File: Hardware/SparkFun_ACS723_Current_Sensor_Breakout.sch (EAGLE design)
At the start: 19 parts, among them J1 455-1750-1-ND, U1 ACS723

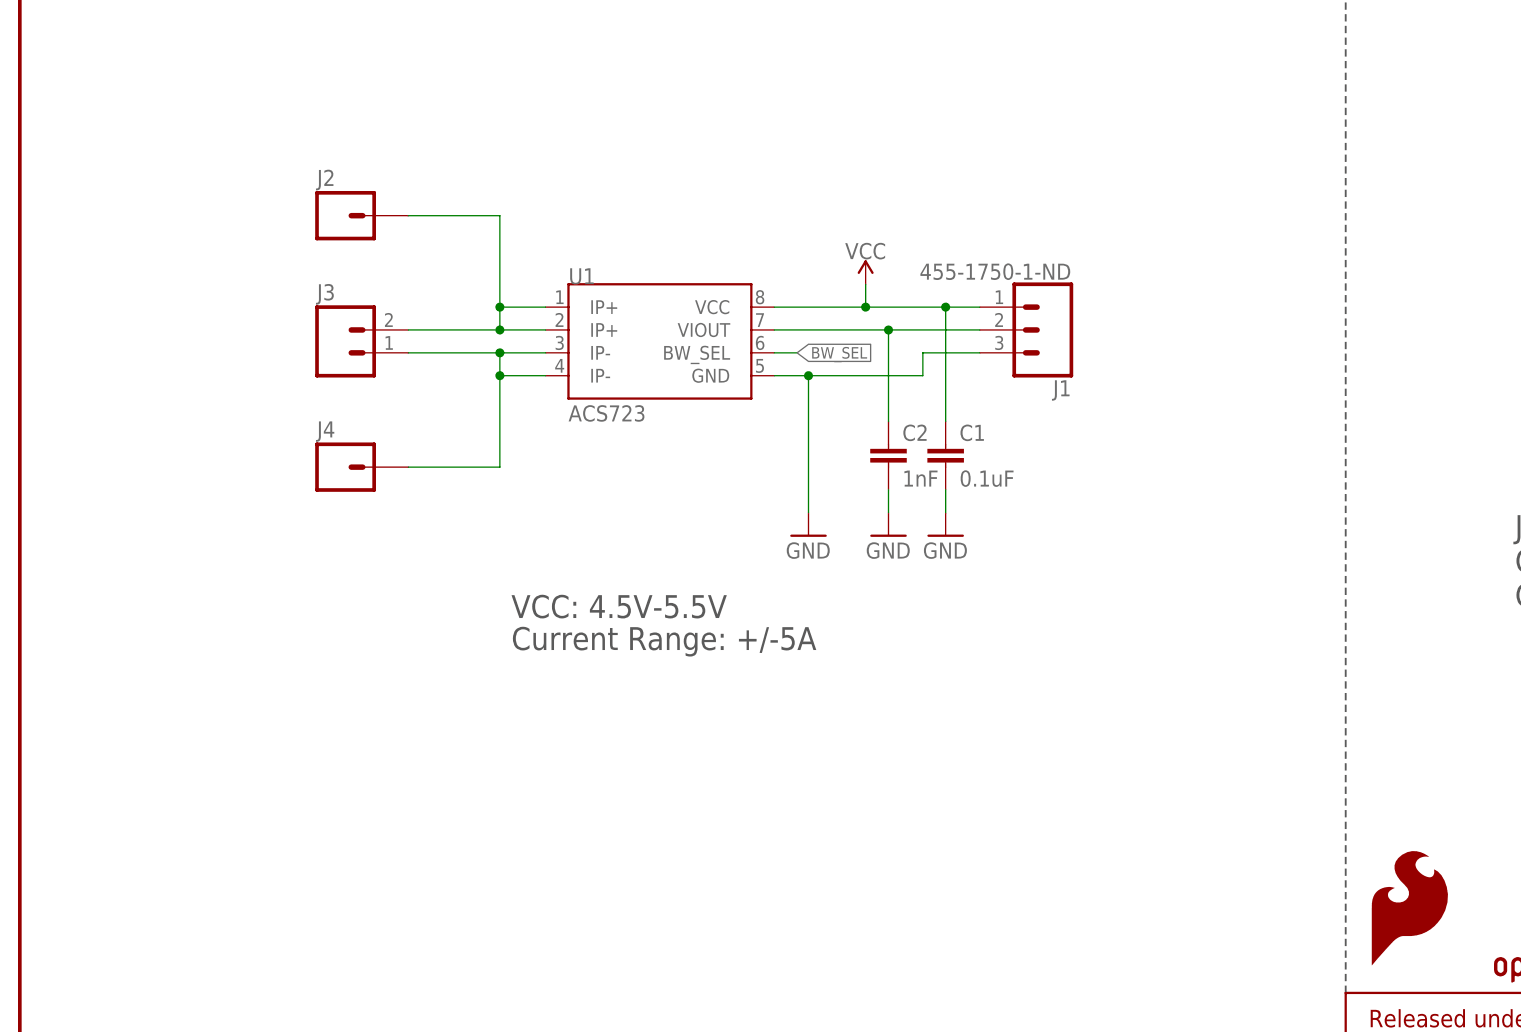
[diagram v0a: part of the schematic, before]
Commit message: removed old design files
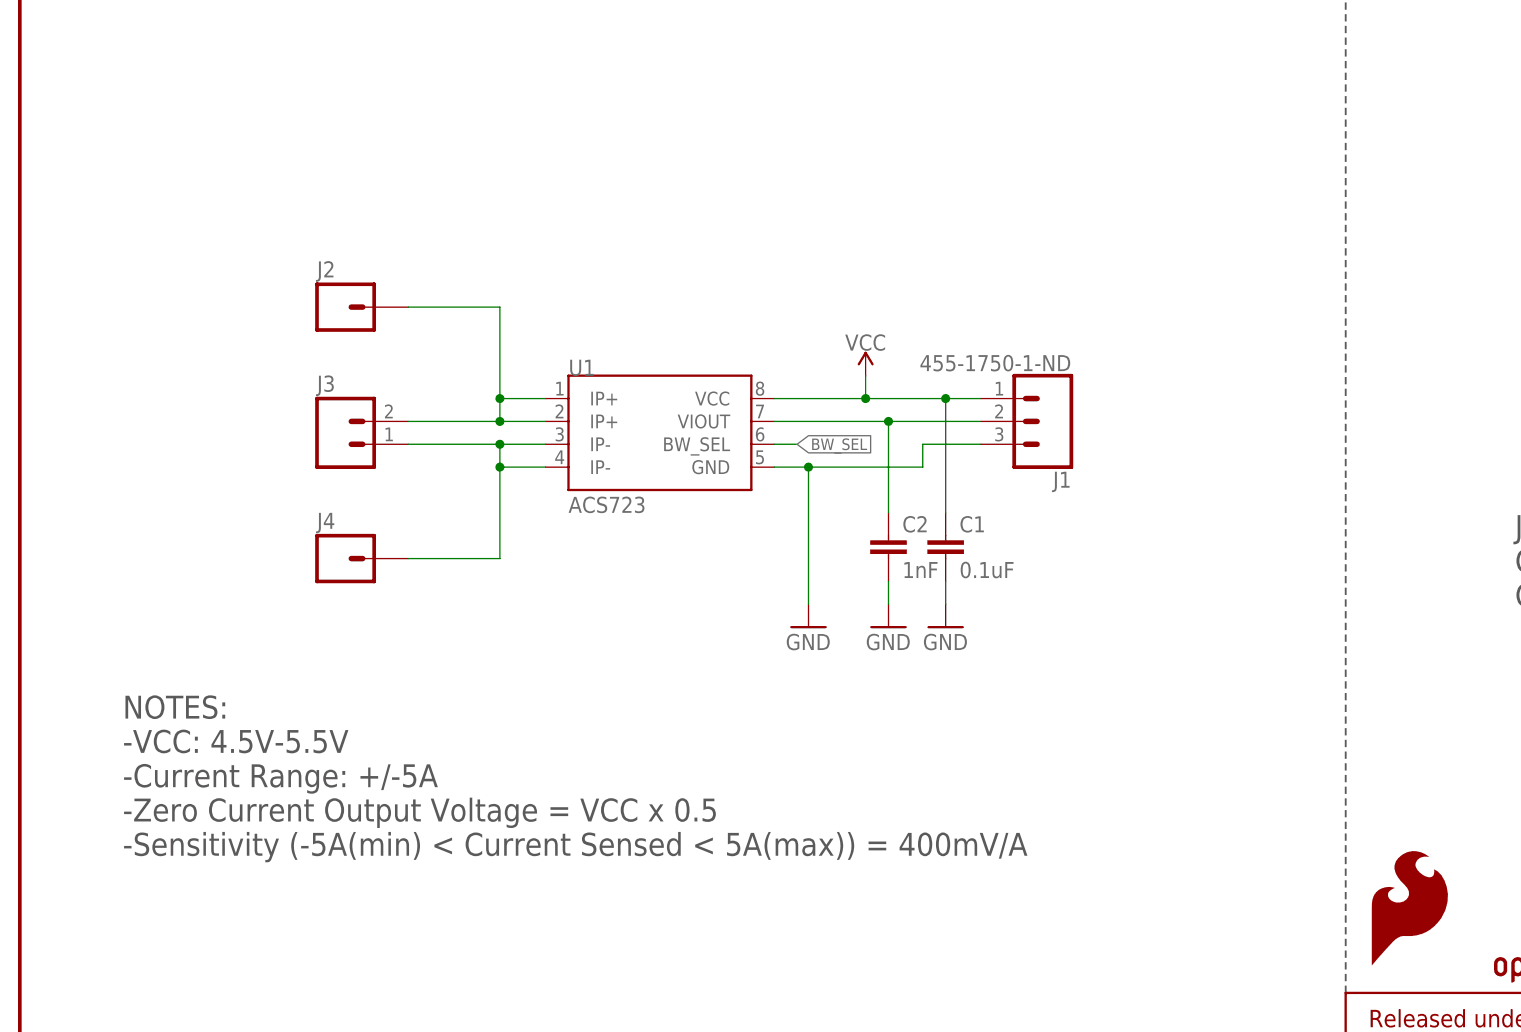
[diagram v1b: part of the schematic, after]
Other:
- note added: "-Current Range: +/-5A"
- note added: "-Sensitivity (-5A(min) < Current Sensed < 5A(max)) = 400mV/A"
- note added: "-VCC: 4.5V-5.5V"
- note added: "-Zero Current Output Voltage = VCC x 0.5"
- note added: "NOTES:"
- note removed: "Current Range: +/-5A"
- note removed: "VCC: 4.5V-5.5V"
- moved on the sheet: C1, C2, J1, J2, J3, J4, U1
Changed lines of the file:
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@@
 <text x="236.982" y="7.366" size="2.54" layer="94">v10</text>
 <text x="175.26" y="6.604" size="2.54" layer="94">Eric Orosel</text>
-<text x="54.61" y="73.66" size="2.54" layer="97">Current Range: +/-5A</text>
-<text x="54.61" y="77.216" size="2.54" layer="97">VCC: 4.5V-5.5V</text>
+<text x="11.43" y="58.42" size="2.54" layer="97">-Current Range: +/-5A</text>
+<text x="11.43" y="62.23" size="2.54" layer="97">-VCC: 4.5V-5.5V</text>
 <text x="166.116" y="86.106" size="2.54" layer="97">JP1 (Sets bandwidth):</text>
 <text x="166.116" y="78.486" size="2.54" layer="97">CLOSED = 80kHz</text>
@@
 <text x="2.286" y="180.34" size="2.54" layer="97">ACS723LLCTR-05AB-T2</text>
 <text x="149.606" y="180.34" size="2.54" layer="97">Bandwidth Select</text>
+<text x="11.43" y="54.61" size="2.54" layer="97">-Zero Current Output Voltage = VCC x 0.5</text>
+<text x="11.43" y="50.8" size="2.54" layer="97">-Sensitivity (-5A(min) &lt; Current Sensed &lt; 5A(max)) = 400mV/A</text>
+<text x="11.43" y="66.04" size="2.54" layer="97">NOTES:</text>
 </plain>
 <instances>
-<instance part="J2" gate="G$1" x="35.56" y="121.92"/>
-<instance part="J4" gate="G$1" x="35.56" y="93.98"/>
-<instance part="J3" gate="G$1" x="35.56" y="106.68"/>
-<instance part="SUPPLY1" gate="G$1" x="93.98" y="114.3"/>
-<instance part="GND1" gate="1" x="87.63" y="86.36"/>
+<instance part="J2" gate="G$1" x="35.56" y="111.76"/>
+<instance part="J4" gate="G$1" x="35.56" y="83.82"/>
+<instance part="J3" gate="G$1" x="35.56" y="96.52"/>
+<instance part="SUPPLY1" gate="G$1" x="93.98" y="104.14"/>
+<instance part="GND1" gate="1" x="87.63" y="76.2"/>
 <instance part="U$1" gate="G$1" x="149.098" y="6.858"/>
-<instance part="U1" gate="G$1" x="71.12" y="106.68"/>
-<instance part="C1" gate="G$1" x="102.87" y="93.98"/>
-<instance part="GND2" gate="1" x="102.87" y="86.36"/>
+<instance part="U1" gate="G$1" x="71.12" y="96.52"/>
+<instance part="C1" gate="G$1" x="102.87" y="83.82"/>
+<instance part="GND2" gate="1" x="102.87" y="76.2"/>
 <instance part="FD2" gate="G$1" x="246.38" y="30.48"/>
 <instance part="FD3" gate="G$1" x="241.3" y="30.48"/>
@@
 <instance part="R1" gate="G$1" x="196.85" y="127" rot="R90"/>
 <instance part="SUPPLY2" gate="G$1" x="196.85" y="134.62"/>
-<instance part="C2" gate="G$1" x="96.52" y="93.98"/>
-<instance part="GND3" gate="1" x="96.52" y="86.36"/>
+<instance part="C2" gate="G$1" x="96.52" y="83.82"/>
+<instance part="GND3" gate="1" x="96.52" y="76.2"/>
 <instance part="FRAME1" gate="G$1" x="0" y="0"/>
 <instance part="FRAME1" gate="V" x="147.32" y="0"/>
-<instance part="J1" gate="J$1" x="114.3" y="109.22" rot="R180"/>
+<instance part="J1" gate="J$1" x="114.3" y="99.06" rot="R180"/>
 <instance part="JP3" gate="G$1" x="236.22" y="25.4"/>
 <instance part="LOGO1" gate="G$1" x="149.86" y="38.1"/>
@@
 <net name="IP+" class="0">
 <segment>
-<wire x1="43.18" y1="121.92" x2="53.34" y2="121.92" width="0.1524" layer="91"/>
-<wire x1="53.34" y1="121.92" x2="53.34" y2="111.76" width="0.1524" layer="91"/>
-<wire x1="53.34" y1="111.76" x2="58.42" y2="111.76" width="0.1524" layer="91"/>
-<wire x1="58.42" y1="109.22" x2="53.34" y2="109.22" width="0.1524" layer="91"/>
-<wire x1="53.34" y1="109.22" x2="53.34" y2="111.76" width="0.1524" layer="91"/>
-<junction x="53.34" y="111.76"/>
+<wire x1="43.18" y1="111.76" x2="53.34" y2="111.76" width="0.1524" layer="91"/>
+<wire x1="53.34" y1="111.76" x2="53.34" y2="101.6" width="0.1524" layer="91"/>
+<wire x1="53.34" y1="101.6" x2="58.42" y2="101.6" width="0.1524" layer="91"/>
+<wire x1="58.42" y1="99.06" x2="53.34" y2="99.06" width="0.1524" layer="91"/>
+<wire x1="53.34" y1="99.06" x2="53.34" y2="101.6" width="0.1524" layer="91"/>
+<junction x="53.34" y="101.6"/>
 <pinref part="J2" gate="G$1" pin="1"/>
 <pinref part="J3" gate="G$1" pin="2"/>
-<wire x1="43.18" y1="109.22" x2="53.34" y2="109.22" width="0.1524" layer="91"/>
-<junction x="53.34" y="109.22"/>
+<wire x1="43.18" y1="99.06" x2="53.34" y2="99.06" width="0.1524" layer="91"/>
+<junction x="53.34" y="99.06"/>
 <pinref part="U1" gate="G$1" pin="IP+@1"/>
 <pinref part="U1" gate="G$1" pin="IP+@2"/>
@@
 <net name="IP-" class="0">
 <segment>
-<wire x1="58.42" y1="106.68" x2="53.34" y2="106.68" width="0.1524" layer="91"/>
-<wire x1="53.34" y1="106.68" x2="53.34" y2="104.14" width="0.1524" layer="91"/>
-<wire x1="53.34" y1="104.14" x2="53.34" y2="93.98" width="0.1524" layer="91"/>
-<wire x1="53.34" y1="93.98" x2="43.18" y2="93.98" width="0.1524" layer="91"/>
-<wire x1="58.42" y1="104.14" x2="53.34" y2="104.14" width="0.1524" layer="91"/>
-<junction x="53.34" y="104.14"/>
+<wire x1="58.42" y1="96.52" x2="53.34" y2="96.52" width="0.1524" layer="91"/>
+<wire x1="53.34" y1="96.52" x2="53.34" y2="93.98" width="0.1524" layer="91"/>
+<wire x1="53.34" y1="93.98" x2="53.34" y2="83.82" width="0.1524" layer="91"/>
+<wire x1="53.34" y1="83.82" x2="43.18" y2="83.82" width="0.1524" layer="91"/>
+<wire x1="58.42" y1="93.98" x2="53.34" y2="93.98" width="0.1524" layer="91"/>
+<junction x="53.34" y="93.98"/>
 <pinref part="J4" gate="G$1" pin="1"/>
 <pinref part="J3" gate="G$1" pin="1"/>
-<wire x1="43.18" y1="106.68" x2="53.34" y2="106.68" width="0.1524" layer="91"/>
-<junction x="53.34" y="106.68"/>
+<wire x1="43.18" y1="96.52" x2="53.34" y2="96.52" width="0.1524" layer="91"/>
+<junction x="53.34" y="96.52"/>
 <pinref part="U1" gate="G$1" pin="IP-@2"/>
 <pinref part="U1" gate="G$1" pin="IP-@1"/>
@@
 <net name="VCC" class="3">
 <segment>
-<wire x1="93.98" y1="111.76" x2="93.98" y2="114.3" width="0.1524" layer="91"/>
+<wire x1="93.98" y1="101.6" x2="93.98" y2="104.14" width="0.1524" layer="91"/>
 <pinref part="SUPPLY1" gate="G$1" pin="VCC"/>
 <pinref part="C1" gate="G$1" pin="1"/>
-<wire x1="102.87" y1="99.06" x2="102.87" y2="111.76" width="0.1524" layer="91"/>
-<junction x="93.98" y="111.76"/>
+<wire x1="102.87" y1="88.9" x2="102.87" y2="101.6" width="0.1524" layer="91"/>
+<junction x="93.98" y="101.6"/>
 <pinref part="U1" gate="G$1" pin="VCC"/>
-<wire x1="102.87" y1="111.76" x2="106.68" y2="111.76" width="0.1524" layer="91"/>
-<wire x1="83.82" y1="111.76" x2="93.98" y2="111.76" width="0.1524" layer="91"/>
-<junction x="102.87" y="111.76"/>
-<wire x1="93.98" y1="111.76" x2="102.87" y2="111.76" width="0.1524" layer="91"/>
+<wire x1="102.87" y1="101.6" x2="106.68" y2="101.6" width="0.1524" layer="91"/>
+<wire x1="83.82" y1="101.6" x2="93.98" y2="101.6" width="0.1524" layer="91"/>
+<junction x="102.87" y="101.6"/>
+<wire x1="93.98" y1="101.6" x2="102.87" y2="101.6" width="0.1524" layer="91"/>
 <pinref part="J1" gate="J$1" pin="1"/>
 </segment>
@@
 <net name="GND" class="3">
 <segment>
-<wire x1="87.63" y1="104.14" x2="87.63" y2="88.9" width="0.1524" layer="91"/>
+<wire x1="87.63" y1="93.98" x2="87.63" y2="78.74" width="0.1524" layer="91"/>
 <pinref part="GND1" gate="1" pin="GND"/>
-<wire x1="87.63" y1="104.14" x2="100.33" y2="104.14" width="0.1524" layer="91"/>
+<wire x1="87.63" y1="93.98" x2="100.33" y2="93.98" width="0.1524" layer="91"/>
 <pinref part="U1" gate="G$1" pin="GND"/>
-<wire x1="87.63" y1="104.14" x2="83.82" y2="104.14" width="0.1524" layer="91"/>
-<junction x="87.63" y="104.14"/>
-<wire x1="100.33" y1="104.14" x2="100.33" y2="106.68" width="0.1524" layer="91"/>
+<wire x1="87.63" y1="93.98" x2="83.82" y2="93.98" width="0.1524" layer="91"/>
+<junction x="87.63" y="93.98"/>
+<wire x1="100.33" y1="93.98" x2="100.33" y2="96.52" width="0.1524" layer="91"/>
 <pinref part="J1" gate="J$1" pin="3"/>
-<wire x1="100.33" y1="106.68" x2="106.68" y2="106.68" width="0.1524" layer="91"/>
+<wire x1="100.33" y1="96.52" x2="106.68" y2="96.52" width="0.1524" layer="91"/>
 </segment>
 <segment>
 <pinref part="C1" gate="G$1" pin="2"/>
-<wire x1="102.87" y1="91.44" x2="102.87" y2="88.9" width="0.1524" layer="91"/>
+<wire x1="102.87" y1="81.28" x2="102.87" y2="78.74" width="0.1524" layer="91"/>
 <pinref part="GND2" gate="1" pin="GND"/>
 </segment>
 <segment>
 <pinref part="C2" gate="G$1" pin="2"/>
-<wire x1="96.52" y1="91.44" x2="96.52" y2="88.9" width="0.1524" layer="91"/>
+<wire x1="96.52" y1="81.28" x2="96.52" y2="78.74" width="0.1524" layer="91"/>
 <pinref part="GND3" gate="1" pin="GND"/>
 </segment>
@@
 <segment>
 <pinref part="U1" gate="G$1" pin="VIOUT"/>
-<wire x1="83.82" y1="109.22" x2="96.52" y2="109.22" width="0.1524" layer="91"/>
-<wire x1="96.52" y1="109.22" x2="106.68" y2="109.22" width="0.1524" layer="91"/>
-<wire x1="96.52" y1="109.22" x2="96.52" y2="99.06" width="0.1524" layer="91"/>
-<junction x="96.52" y="109.22"/>
+<wire x1="83.82" y1="99.06" x2="96.52" y2="99.06" width="0.1524" layer="91"/>
+<wire x1="96.52" y1="99.06" x2="106.68" y2="99.06" width="0.1524" layer="91"/>
+<wire x1="96.52" y1="99.06" x2="96.52" y2="88.9" width="0.1524" layer="91"/>
+<junction x="96.52" y="99.06"/>
 <pinref part="C2" gate="G$1" pin="1"/>
 <pinref part="J1" gate="J$1" pin="2"/>
@@
 <segment>
 <pinref part="U1" gate="G$1" pin="BW_SEL"/>
-<wire x1="83.82" y1="106.68" x2="86.36" y2="106.68" width="0.1524" layer="91"/>
-<label x="86.36" y="106.68" size="1.27" layer="95" xref="yes"/>
+<wire x1="83.82" y1="96.52" x2="86.36" y2="96.52" width="0.1524" layer="91"/>
+<label x="86.36" y="96.52" size="1.27" layer="95" xref="yes"/>
 </segment>
 <segment>
